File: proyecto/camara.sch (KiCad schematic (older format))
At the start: 19 parts, among them J6 USB_A, J7 AVR-JTAG-10, SW2 SW_Push, U6 Omega2+

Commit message: Add files via upload
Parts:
- D4: footprint Diode_THT:D_DO-41_SOD81_P10.16mm_Horizontal -> Diode_THT:D_DO-41_SOD81_P5.08mm_Vertical_AnodeUp
- SW2: footprint Button_Switch_SMD:SW_DIP_SPSTx01_Slide_6.7x4.1mm_W6.73mm_P2.54mm_LowProfile_JPin -> Button_Switch_SMD:SW_Push_1P1T_NO_6x6mm_H9.5mm
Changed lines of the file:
@@
 F 0 "SW2" V 8546 5352 50  0000 R CNN
 F 1 "SW_Push" V 8455 5352 50  0000 R CNN
-F 2 "Button_Switch_SMD:SW_DIP_SPSTx01_Slide_6.7x4.1mm_W6.73mm_P2.54mm_LowProfile_JPin" H 8500 5600 50  0001 C CNN
+F 2 "Button_Switch_SMD:SW_Push_1P1T_NO_6x6mm_H9.5mm" H 8500 5600 50  0001 C CNN
 F 3 "~" H 8500 5600 50  0001 C CNN
 	1    8500 5400
@@
 F 0 "D4" V 2704 1479 50  0000 L CNN
 F 1 "1N47xxA" V 2795 1479 50  0000 L CNN
-F 2 "Diode_THT:D_DO-41_SOD81_P10.16mm_Horizontal" H 2750 1225 50  0001 C CNN
+F 2 "Diode_THT:D_DO-41_SOD81_P5.08mm_Vertical_AnodeUp" H 2750 1225 50  0001 C CNN
 F 3 "https://www.vishay.com/docs/85816/1n4728a.pdf" H 2750 1400 50  0001 C CNN
 	1    2750 1400

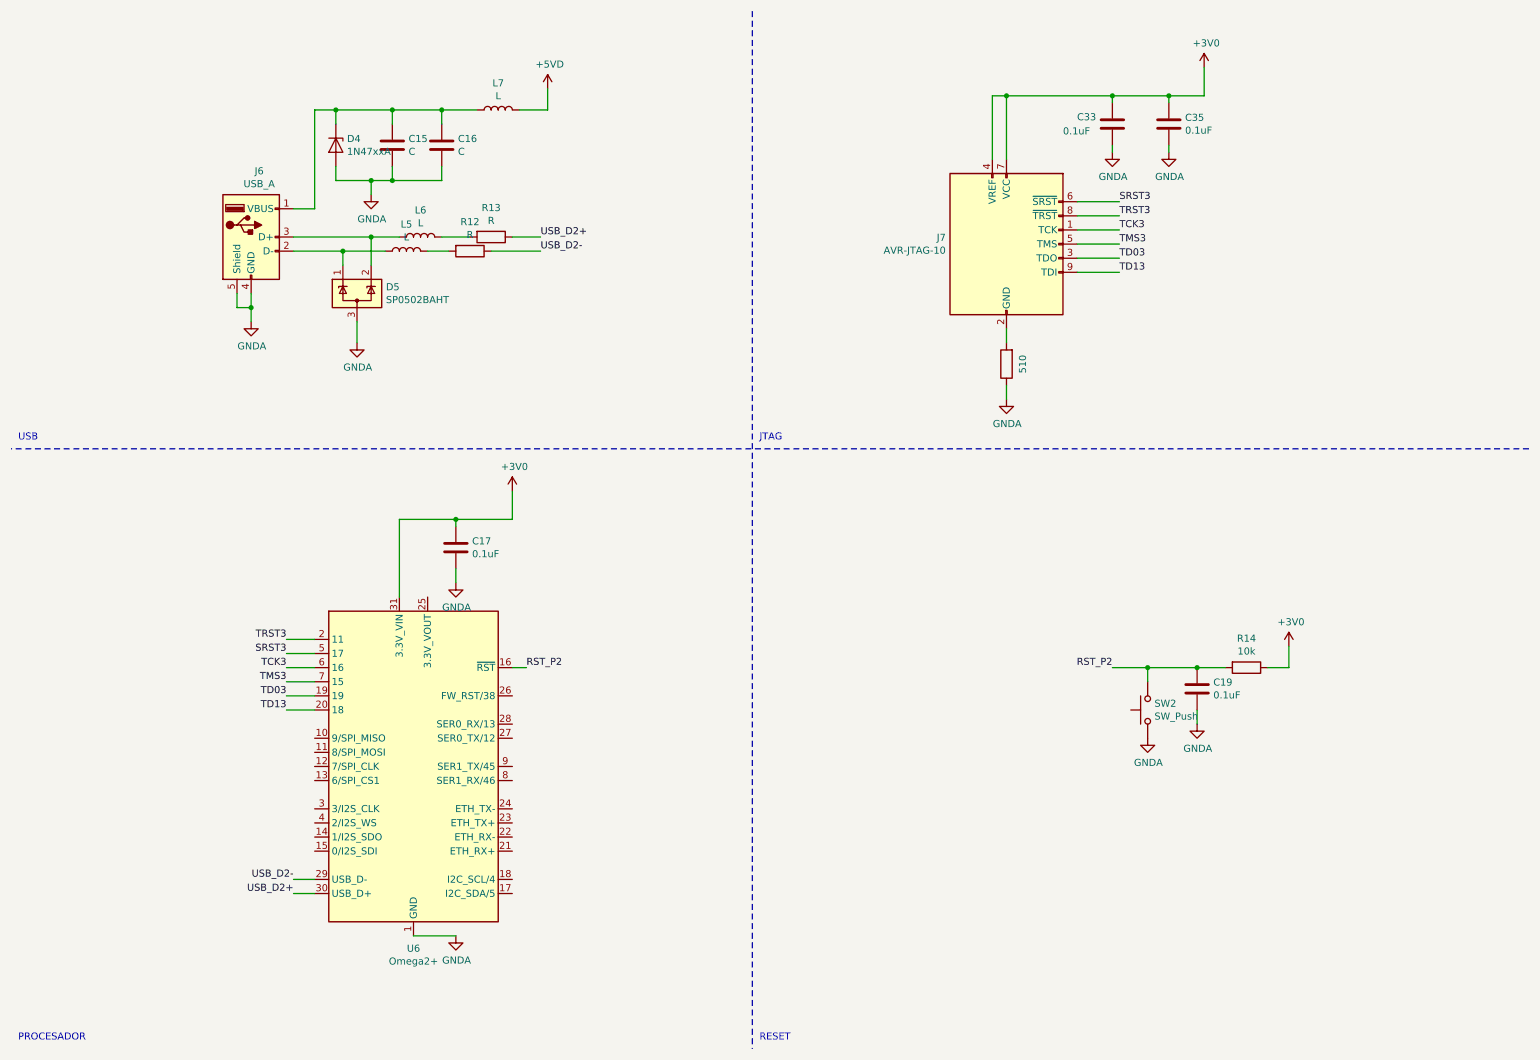
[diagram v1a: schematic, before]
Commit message: Add files via upload
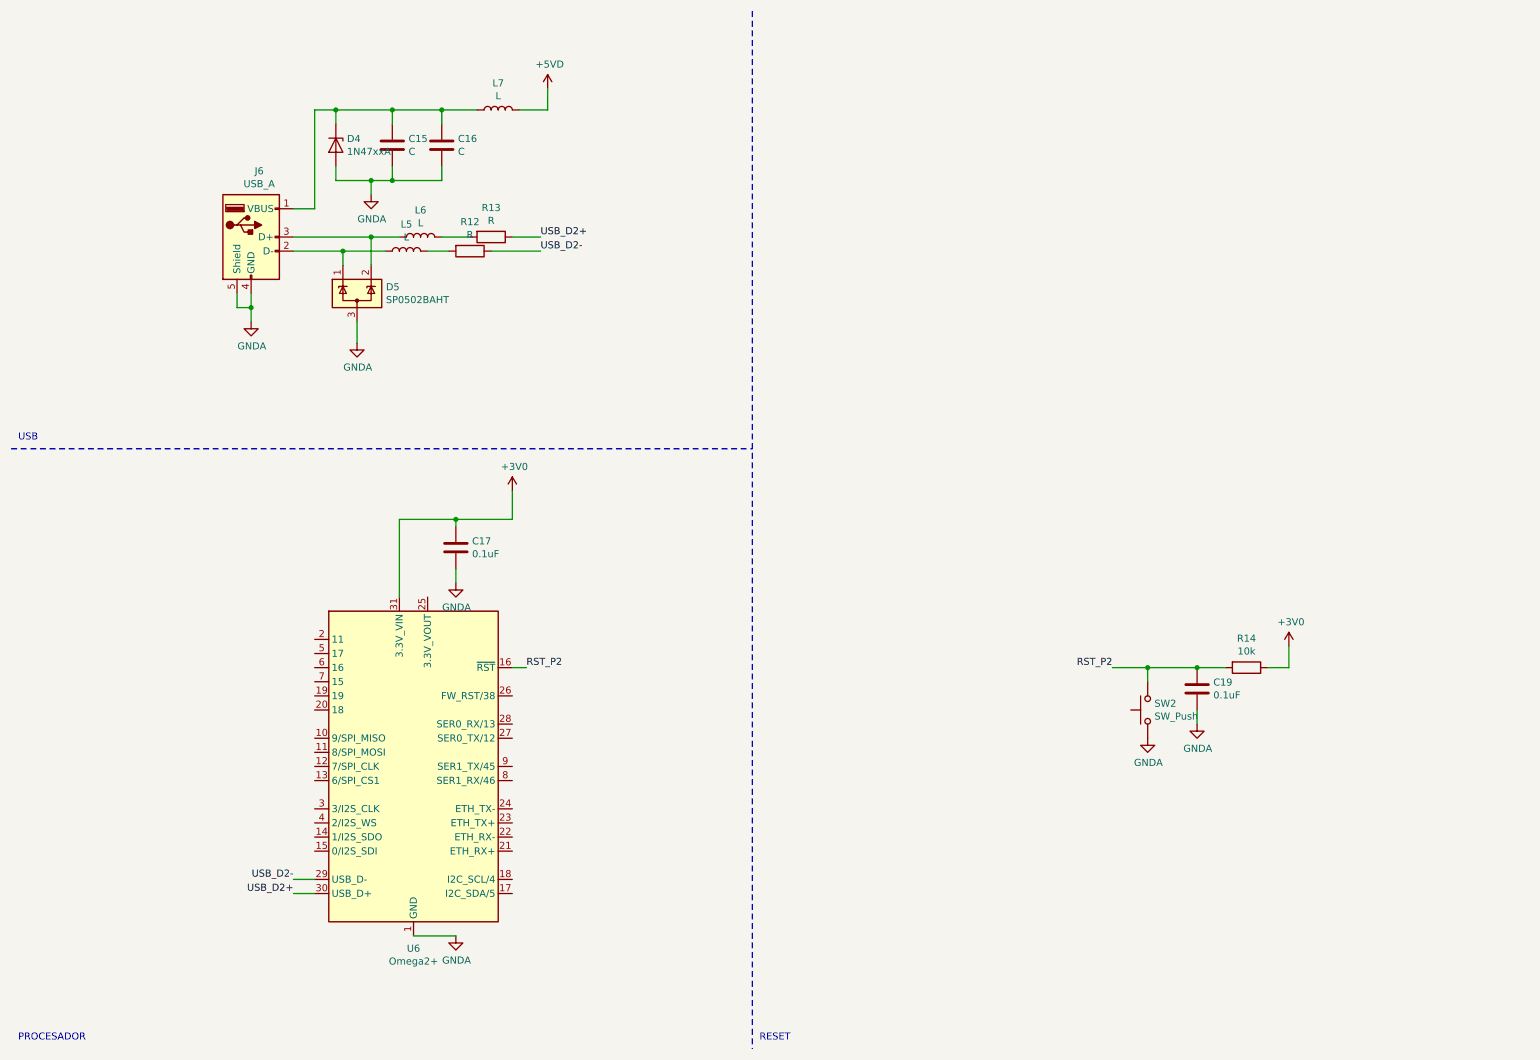
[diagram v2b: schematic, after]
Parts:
- removed C33, C35: 0.1uF, Capacitor_SMD:C_0603_1608Metric_Pad1.05x0.95mm_HandSolder, symbol Device:C
- removed J7: AVR-JTAG-10, Connector_PinSocket_2.54mm:PinSocket_1x10_P2.54mm_Vertical, symbol Connector:AVR-JTAG-10
- removed R15: 510, Resistor_SMD:R_0603_1608Metric_Pad1.05x0.95mm_HandSolder, symbol Device:R
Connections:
- net SRST3: no longer names the net of U6.5 (17)
- net TCK3: no longer names the net of U6.6 (16)
- net TD03: no longer names the net of U6.19
- net TD13: no longer names the net of U6.20 (18)
- net TMS3: no longer names the net of U6.7 (15)
- net TRST3: no longer names the net of U6.2 (11)
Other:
- note removed: "JTAG"
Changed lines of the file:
@@
 $Descr A4 11693 8268
 encoding utf-8
-Sheet 5 7
+Sheet 4 7
 Title ""
 Date ""
@@
 	1    0    0    -1
 $EndComp
-Wire Wire Line
-	8300 2300 8000 2300
-Wire Wire Line
-	8000 2200 8300 2200
-Wire Wire Line
-	8300 2100 8000 2100
-Wire Wire Line
-	7500 3200 7500 3100
-Wire Wire Line
-	8000 2000 8300 2000
-Wire Wire Line
-	8000 1800 8300 1800
-Text Label 8300 2000 0    50   ~ 0
-TCK3
-Text Label 8300 2100 0    50   ~ 0
-TMS3
-Text Label 8300 2200 0    50   ~ 0
-TD03
-Text Label 8300 2300 0    50   ~ 0
-TD13
-$Comp
-L Device:R R?
-U 1 1 5EA69365
-P 7500 2950
-AR Path="/5E9DF408/5EA69365" Ref="R?"  Part="1"
-AR Path="/5E9DF2DA/5EA69365" Ref="R15"  Part="1"
-F 0 "R15" V 7293 2950 50  0001 C CNN
-F 1 "510" V 7385 2950 50  0000 C CNN
-F 2 "Resistor_SMD:R_0603_1608Metric_Pad1.05x0.95mm_HandSolder" V 7430 2950 50  0001 C CNN
-F 3 "~" H 7500 2950 50  0001 C CNN
-	1    7500 2950
-	-1   0    0    1
-$EndComp
 $Comp
 L power:GNDA #PWR0138
@@
 Wire Wire Line
 	4100 5100 4000 5100
-$Comp
-L power:GNDA #PWR0140
-U 1 1 5EA8F42E
-P 7500 3200
-F 0 "#PWR0140" H 7500 2950 50  0001 C CNN
-F 1 "GNDA" H 7505 3027 50  0000 C CNN
-F 2 "" H 7500 3200 50  0001 C CNN
-F 3 "" H 7500 3200 50  0001 C CNN
-	1    7500 3200
-	1    0    0    -1
-$EndComp
-Wire Wire Line
-	2600 4900 2400 4900
-Wire Wire Line
-	2400 5000 2600 5000
-Wire Wire Line
-	2600 5100 2400 5100
-Wire Wire Line
-	2400 5200 2600 5200
-Wire Wire Line
-	2600 5300 2400 5300
-Wire Wire Line
-	2600 5400 2400 5400
-Text Label 2400 5400 2    50   ~ 0
-TD13
-Text Label 2400 5300 2    50   ~ 0
-TD03
-Text Label 2400 5200 2    50   ~ 0
-TMS3
-Text Label 2400 5100 2    50   ~ 0
-TCK3
-Text Label 2400 5000 2    50   ~ 0
-SRST3
-Text Label 2400 4900 2    50   ~ 0
-TRST3
 Wire Notes Line
 	5700 450  5700 7800
-Text Notes 5750 3500 0    50   ~ 0
-JTAG
 Text Notes 5750 7750 0    50   ~ 0
 RESET
@@
 $EndComp
 Wire Notes Line
-	11200 3550 450  3550
-Wire Wire Line
-	8900 850  8900 1050
-Wire Wire Line
-	8650 1450 8650 1400
-Wire Wire Line
-	8900 1050 8650 1050
-Connection ~ 8650 1050
-Wire Wire Line
-	8650 1100 8650 1050
-$Comp
-L Device:C C?
-U 1 1 5EC6B22B
-P 8650 1250
-AR Path="/5EC6B22B" Ref="C?"  Part="1"
-AR Path="/5E9F954D/5EC6B22B" Ref="C?"  Part="1"
-AR Path="/5E9DF2DA/5EC6B22B" Ref="C35"  Part="1"
-F 0 "C35" H 8765 1296 50  0000 L CNN
-F 1 "0.1uF" H 8765 1205 50  0000 L CNN
-F 2 "Capacitor_SMD:C_0603_1608Metric_Pad1.05x0.95mm_HandSolder" H 8688 1100 50  0001 C CNN
-F 3 "~" H 8650 1250 50  0001 C CNN
-	1    8650 1250
-	1    0    0    -1
-$EndComp
-$Comp
-L power:+3V0 #PWR0158
-U 1 1 5EC6B231
-P 8900 850
-F 0 "#PWR0158" H 8900 700 50  0001 C CNN
-F 1 "+3V0" H 8915 1023 50  0000 C CNN
-F 2 "" H 8900 850 50  0001 C CNN
-F 3 "" H 8900 850 50  0001 C CNN
-	1    8900 850
-	1    0    0    -1
-$EndComp
-Wire Wire Line
-	8250 1450 8250 1400
-Wire Wire Line
-	8250 1100 8250 1050
-$Comp
-L Device:C C?
-U 1 1 5EC6E917
-P 8250 1250
-AR Path="/5EC6E917" Ref="C?"  Part="1"
-AR Path="/5E9F954D/5EC6E917" Ref="C?"  Part="1"
-AR Path="/5E9DF2DA/5EC6E917" Ref="C33"  Part="1"
-F 0 "C33" H 8000 1300 50  0000 L CNN
-F 1 "0.1uF" H 7900 1200 50  0000 L CNN
-F 2 "Capacitor_SMD:C_0603_1608Metric_Pad1.05x0.95mm_HandSolder" H 8288 1100 50  0001 C CNN
-F 3 "~" H 8250 1250 50  0001 C CNN
-	1    8250 1250
-	1    0    0    -1
-$EndComp
-Wire Wire Line
-	7500 1050 7500 1500
-Wire Wire Line
-	7500 1050 8250 1050
-Wire Wire Line
-	7400 1500 7400 1050
-Wire Wire Line
-	7400 1050 7500 1050
-Connection ~ 7500 1050
-Connection ~ 8250 1050
-Wire Wire Line
-	8250 1050 8650 1050
-$Comp
-L Connector:AVR-JTAG-10 J7
-U 1 1 5EC90AF4
-P 7500 2100
-F 0 "J7" H 7070 2146 50  0000 R CNN
-F 1 "AVR-JTAG-10" H 7070 2055 50  0000 R CNN
-F 2 "Connector_PinSocket_2.54mm:PinSocket_1x10_P2.54mm_Vertical" V 7350 2250 50  0001 C CNN
-F 3 " ~" H 6225 1550 50  0001 C CNN
-	1    7500 2100
-	1    0    0    -1
-$EndComp
-Wire Wire Line
-	7500 2800 7500 2700
-$Comp
-L power:GNDA #PWR0161
-U 1 1 5EC6E91D
-P 8250 1450
-F 0 "#PWR0161" H 8250 1200 50  0001 C CNN
-F 1 "GNDA" H 8255 1277 50  0000 C CNN
-F 2 "" H 8250 1450 50  0001 C CNN
-F 3 "" H 8250 1450 50  0001 C CNN
-	1    8250 1450
-	1    0    0    -1
-$EndComp
-$Comp
-L power:GNDA #PWR0159
-U 1 1 5EC6B237
-P 8650 1450
-F 0 "#PWR0159" H 8650 1200 50  0001 C CNN
-F 1 "GNDA" H 8655 1277 50  0000 C CNN
-F 2 "" H 8650 1450 50  0001 C CNN
-F 3 "" H 8650 1450 50  0001 C CNN
-	1    8650 1450
-	1    0    0    -1
-$EndComp
-Text Label 8300 1800 0    50   ~ 0
-SRST3
-Text Label 8300 1900 0    50   ~ 0
-TRST3
-Wire Wire Line
-	8000 1900 8300 1900
+	450  3550 5700 3550
 $EndSCHEMATC
